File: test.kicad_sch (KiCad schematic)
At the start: 60 parts, among them J1 USB_C_Receptacle_USB2.0_16P, J2 Conn_01x02_Pin (switch), J3 Conn_01x02_Pin (battery), J4 Conn_01x03_Pin, SW1 SW_Push, SW10 SW_Push, SW11 SW_Push, SW12 SW_Push, SW13 SW_Push, SW14 SW_Push, SW15 SW_Push, SW16 SW_Push, SW17 SW_Push, SW18 SW_Push, SW19 SW_Push, SW2 SW_Push, SW3 SW_Push, SW4 SW_Push, SW5 SW_Push, SW6 SW_Push, SW7 SW_Push, SW8 SW_Push, SW9 SW_Push, U1 E73-2G4M08S1C, U2 AP2112K-3.3, U3 MCP73831-2-OT, U4 USBLC6-2SC6

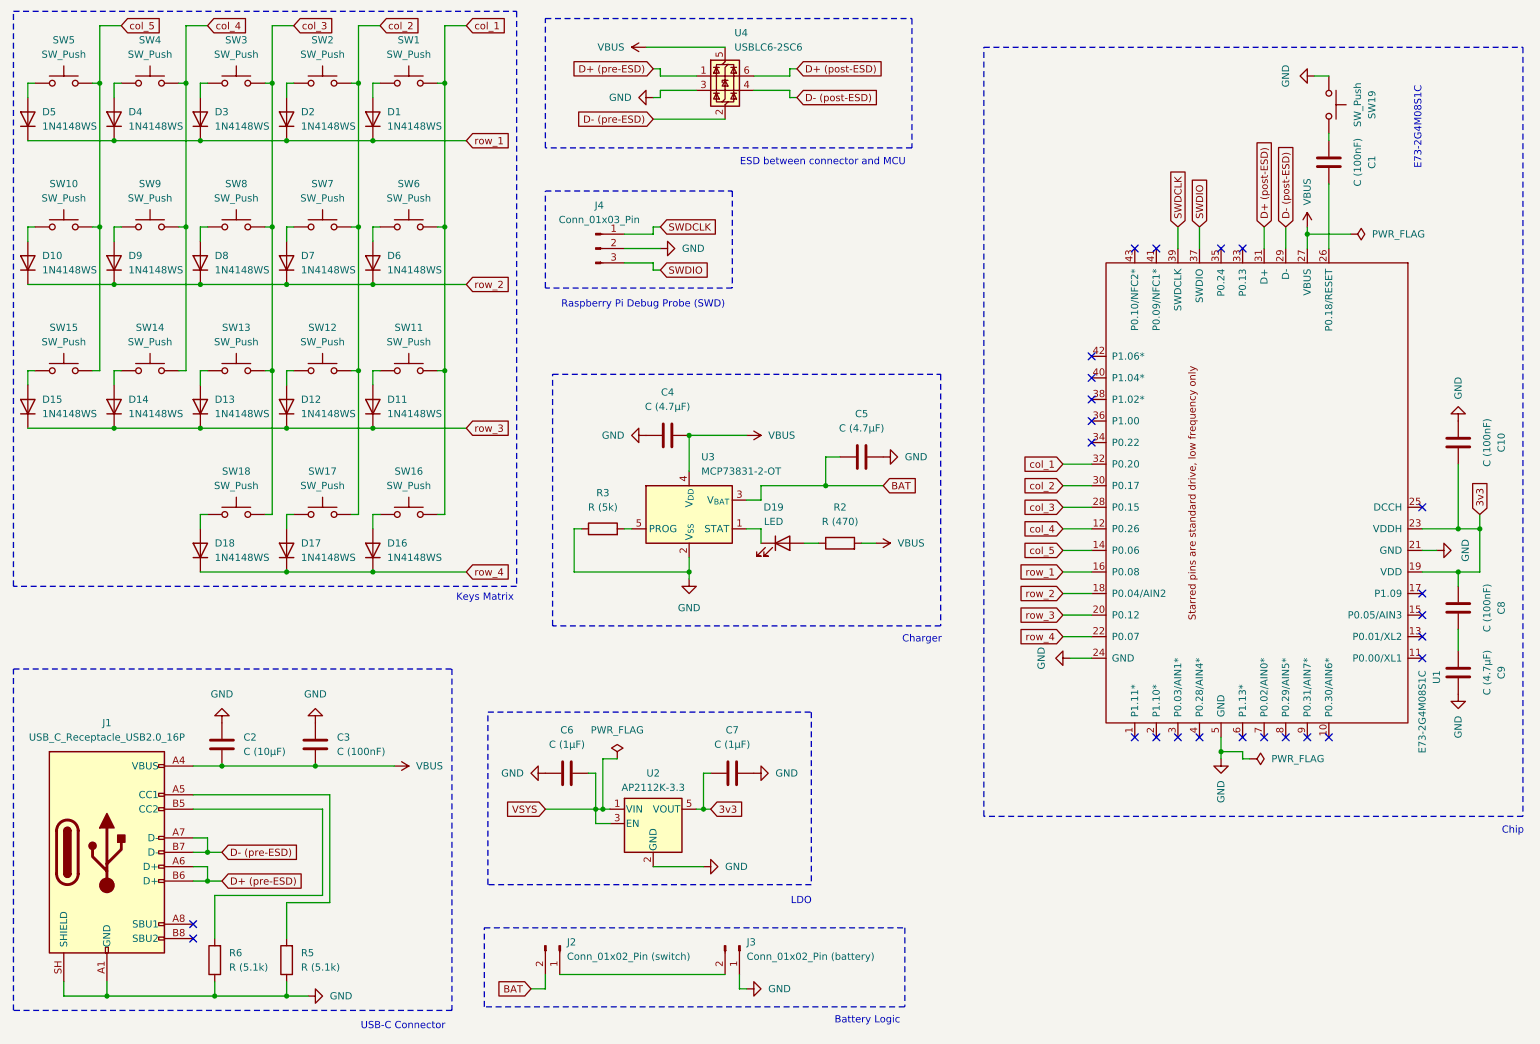
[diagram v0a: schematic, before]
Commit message: feat: init pcb
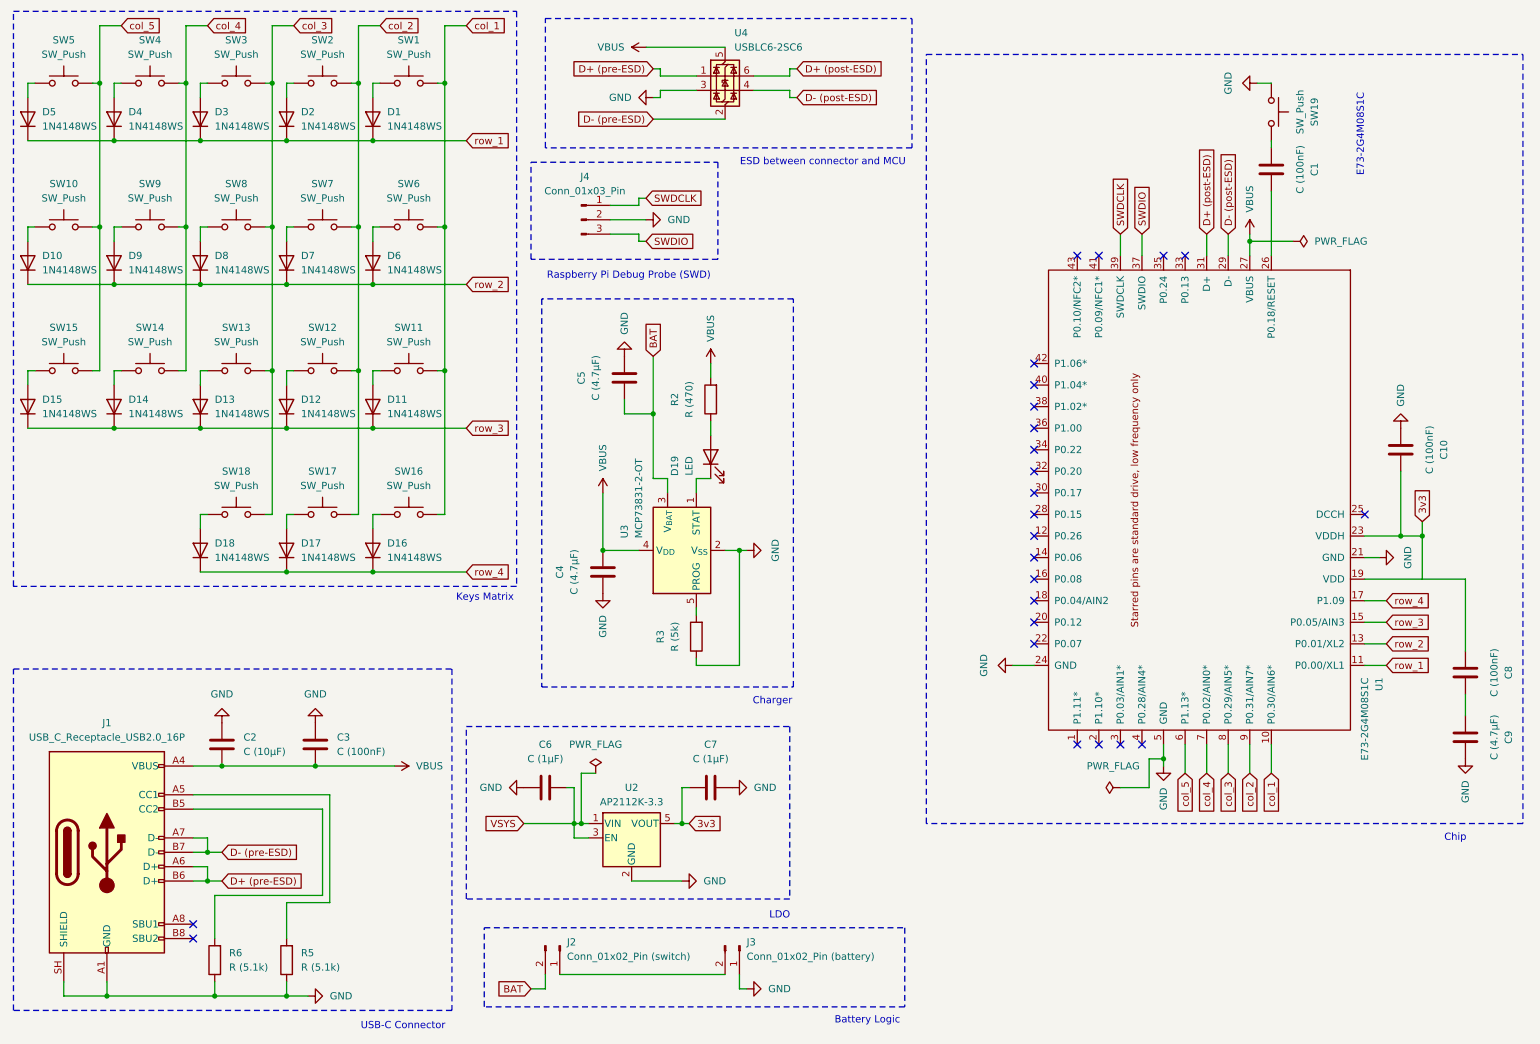
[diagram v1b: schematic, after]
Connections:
- net 3v3: no longer C8.1, U1.19 (VDD)
- net col_1: now also U1.10 (P0.30/AIN6*); no longer U1.32 (P0.20)
- net col_2: now also U1.9 (P0.31/AIN7*); no longer U1.30 (P0.17)
- net col_3: now also U1.8 (P0.29/AIN5*); no longer U1.28 (P0.15)
- net col_4: now also U1.7 (P0.02/AIN0*); no longer U1.12 (P0.26)
- net col_5: now also U1.6 (P1.13*); no longer U1.14 (P0.06)
- net row_1: now also U1.11 (P0.00/XL1); no longer U1.16 (P0.08)
- net row_2: now also U1.13 (P0.01/XL2); no longer U1.18 (P0.04/AIN2)
- net row_3: now also U1.15 (P0.05/AIN3); no longer U1.20 (P0.12)
- net row_4: now also U1.17 (P1.09); no longer U1.22 (P0.07)
- new net: C8.1, U1.19 (VDD)
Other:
- moved on the sheet: C1, C10, C4, C5, C6, C7, C8, C9, D19, J4, R2, R3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

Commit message: feat(pcb): upgrade it
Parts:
- C1, C10, C2, C3, C4, C5, C6, C7, C8, C9: footprint Capacitor_SMD:C_0201_0603Metric -> Capacitor_SMD:C_0805_2012Metric_Pad1.18x1.45mm_HandSolder
- D19: footprint LED_SMD:LED_PLCC-2_3.4x3.0mm_AK -> LED_SMD:LED_0201_0603Metric_Pad0.64x0.40mm_HandSolder
- R2, R3, R5, R6: footprint Resistor_SMD:R_0201_0603Metric -> Resistor_SMD:R_0805_2012Metric_Pad1.20x1.40mm_HandSolder
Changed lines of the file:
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@@
 			)
 		)
-		(property "Footprint" "Capacitor_SMD:C_0201_0603Metric"
+		(property "Footprint" "Capacitor_SMD:C_0805_2012Metric_Pad1.18x1.45mm_HandSolder"
 			(at 53.0352 148.59 0)
 			(hide yes)
@@
 			)
 		)
-		(property "Footprint" "Resistor_SMD:R_0201_0603Metric"
+		(property "Footprint" "Resistor_SMD:R_0805_2012Metric_Pad1.20x1.40mm_HandSolder"
 			(at 140.208 83.82 90)
 			(hide yes)
@@
 			)
 		)
-		(property "Footprint" "Resistor_SMD:R_0201_0603Metric"
+		(property "Footprint" "Resistor_SMD:R_0805_2012Metric_Pad1.20x1.40mm_HandSolder"
 			(at 137.668 125.73 90)
 			(hide yes)
@@
 			)
 		)
-		(property "Footprint" "Capacitor_SMD:C_0201_0603Metric"
+		(property "Footprint" "Capacitor_SMD:C_0805_2012Metric_Pad1.18x1.45mm_HandSolder"
 			(at 261.3152 96.52 0)
 			(hide yes)
@@
 			)
 		)
-		(property "Footprint" "Resistor_SMD:R_0201_0603Metric"
+		(property "Footprint" "Resistor_SMD:R_0805_2012Metric_Pad1.20x1.40mm_HandSolder"
 			(at 65.278 182.88 90)
 			(hide yes)
@@
 			)
 		)
-		(property "Footprint" "Capacitor_SMD:C_0201_0603Metric"
+		(property "Footprint" "Capacitor_SMD:C_0805_2012Metric_Pad1.18x1.45mm_HandSolder"
 			(at 142.24 151.4348 0)
 			(hide yes)
@@
 			)
 		)
-		(property "Footprint" "Capacitor_SMD:C_0201_0603Metric"
+		(property "Footprint" "Capacitor_SMD:C_0805_2012Metric_Pad1.18x1.45mm_HandSolder"
 			(at 272.7452 135.89 0)
 			(hide yes)
@@
 			)
 		)
-		(property "Footprint" "Capacitor_SMD:C_0201_0603Metric"
+		(property "Footprint" "Capacitor_SMD:C_0805_2012Metric_Pad1.18x1.45mm_HandSolder"
 			(at 113.03 151.4348 0)
 			(hide yes)
@@
 			)
 		)
-		(property "Footprint" "Resistor_SMD:R_0201_0603Metric"
+		(property "Footprint" "Resistor_SMD:R_0805_2012Metric_Pad1.20x1.40mm_HandSolder"
 			(at 52.578 182.88 90)
 			(hide yes)
@@
 			)
 		)
-		(property "Footprint" "Capacitor_SMD:C_0201_0603Metric"
+		(property "Footprint" "Capacitor_SMD:C_0805_2012Metric_Pad1.18x1.45mm_HandSolder"
 			(at 238.4552 46.99 0)
 			(hide yes)
@@
 			)
 		)
-		(property "Footprint" "LED_SMD:LED_PLCC-2_3.4x3.0mm_AK"
+		(property "Footprint" "LED_SMD:LED_0201_0603Metric_Pad0.64x0.40mm_HandSolder"
 			(at 138.43 93.98 0)
 			(hide yes)
@@
 			)
 		)
-		(property "Footprint" "Capacitor_SMD:C_0201_0603Metric"
+		(property "Footprint" "Capacitor_SMD:C_0805_2012Metric_Pad1.18x1.45mm_HandSolder"
 			(at 69.5452 148.59 0)
 			(hide yes)
@@
 			)
 		)
-		(property "Footprint" "Capacitor_SMD:C_0201_0603Metric"
+		(property "Footprint" "Capacitor_SMD:C_0805_2012Metric_Pad1.18x1.45mm_HandSolder"
 			(at 272.7452 147.32 0)
 			(hide yes)
@@
 			)
 		)
-		(property "Footprint" "Capacitor_SMD:C_0201_0603Metric"
+		(property "Footprint" "Capacitor_SMD:C_0805_2012Metric_Pad1.18x1.45mm_HandSolder"
 			(at 122.2248 76.2 0)
 			(hide yes)
@@
 			)
 		)
-		(property "Footprint" "Capacitor_SMD:C_0201_0603Metric"
+		(property "Footprint" "Capacitor_SMD:C_0805_2012Metric_Pad1.18x1.45mm_HandSolder"
 			(at 118.4148 110.49 0)
 			(hide yes)
